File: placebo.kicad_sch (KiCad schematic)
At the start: 15 parts

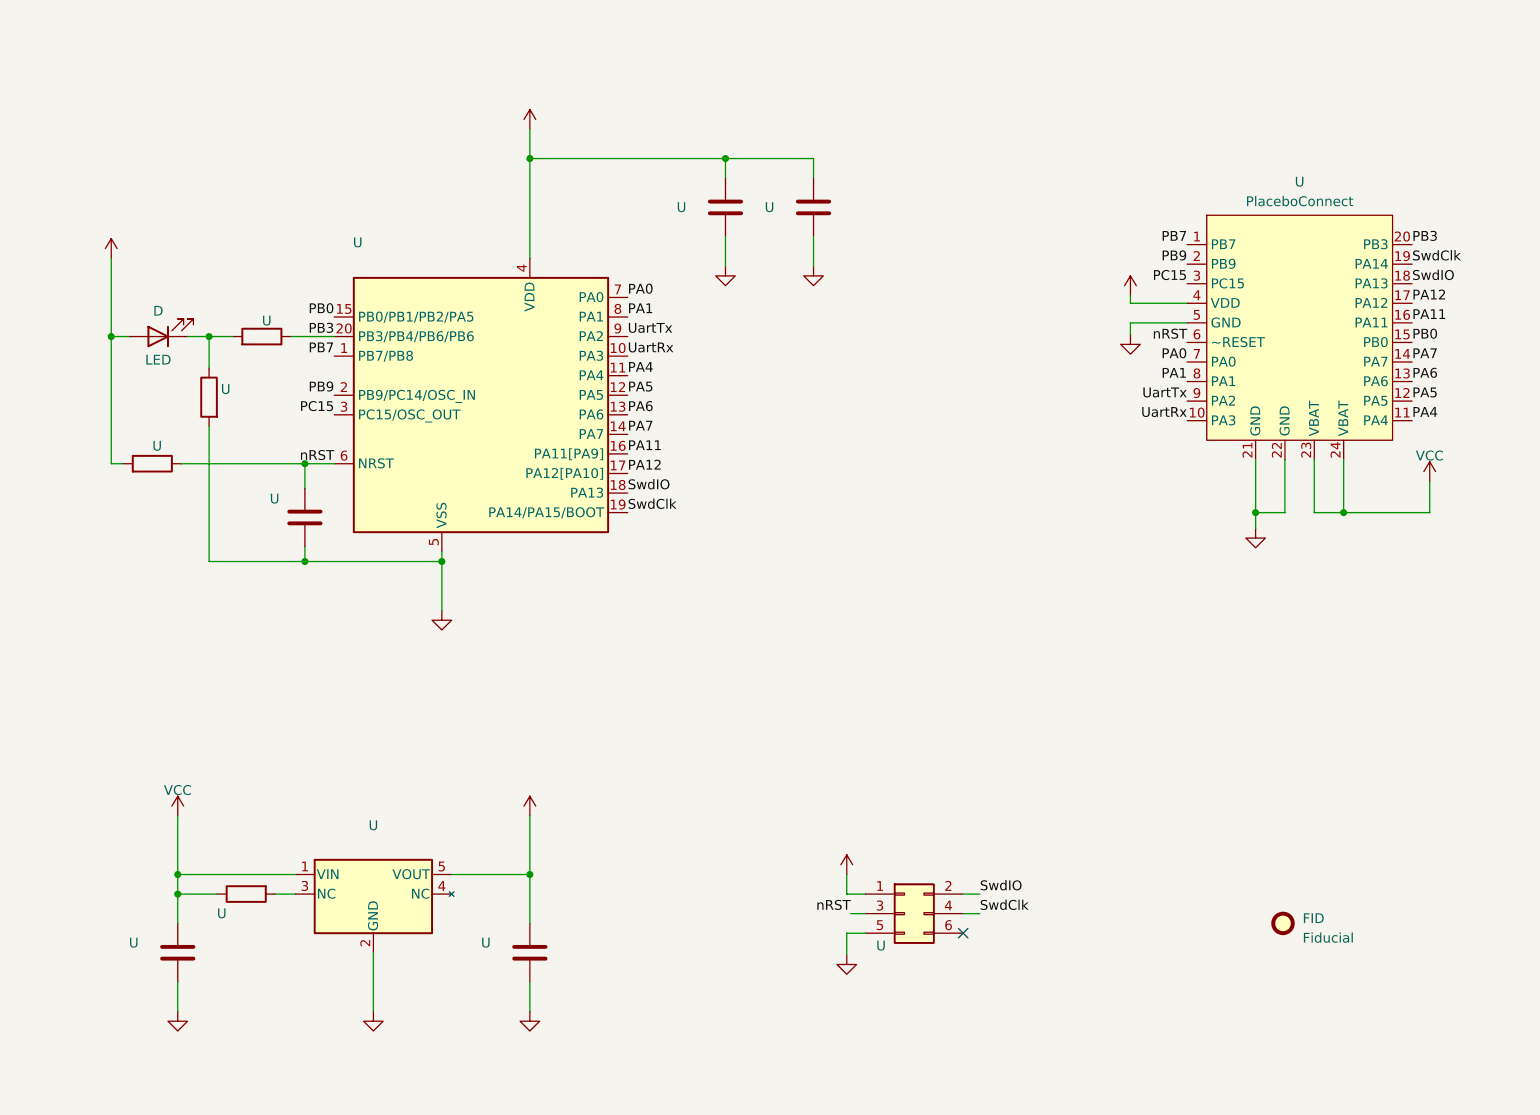
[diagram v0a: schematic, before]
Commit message: rev.0x7
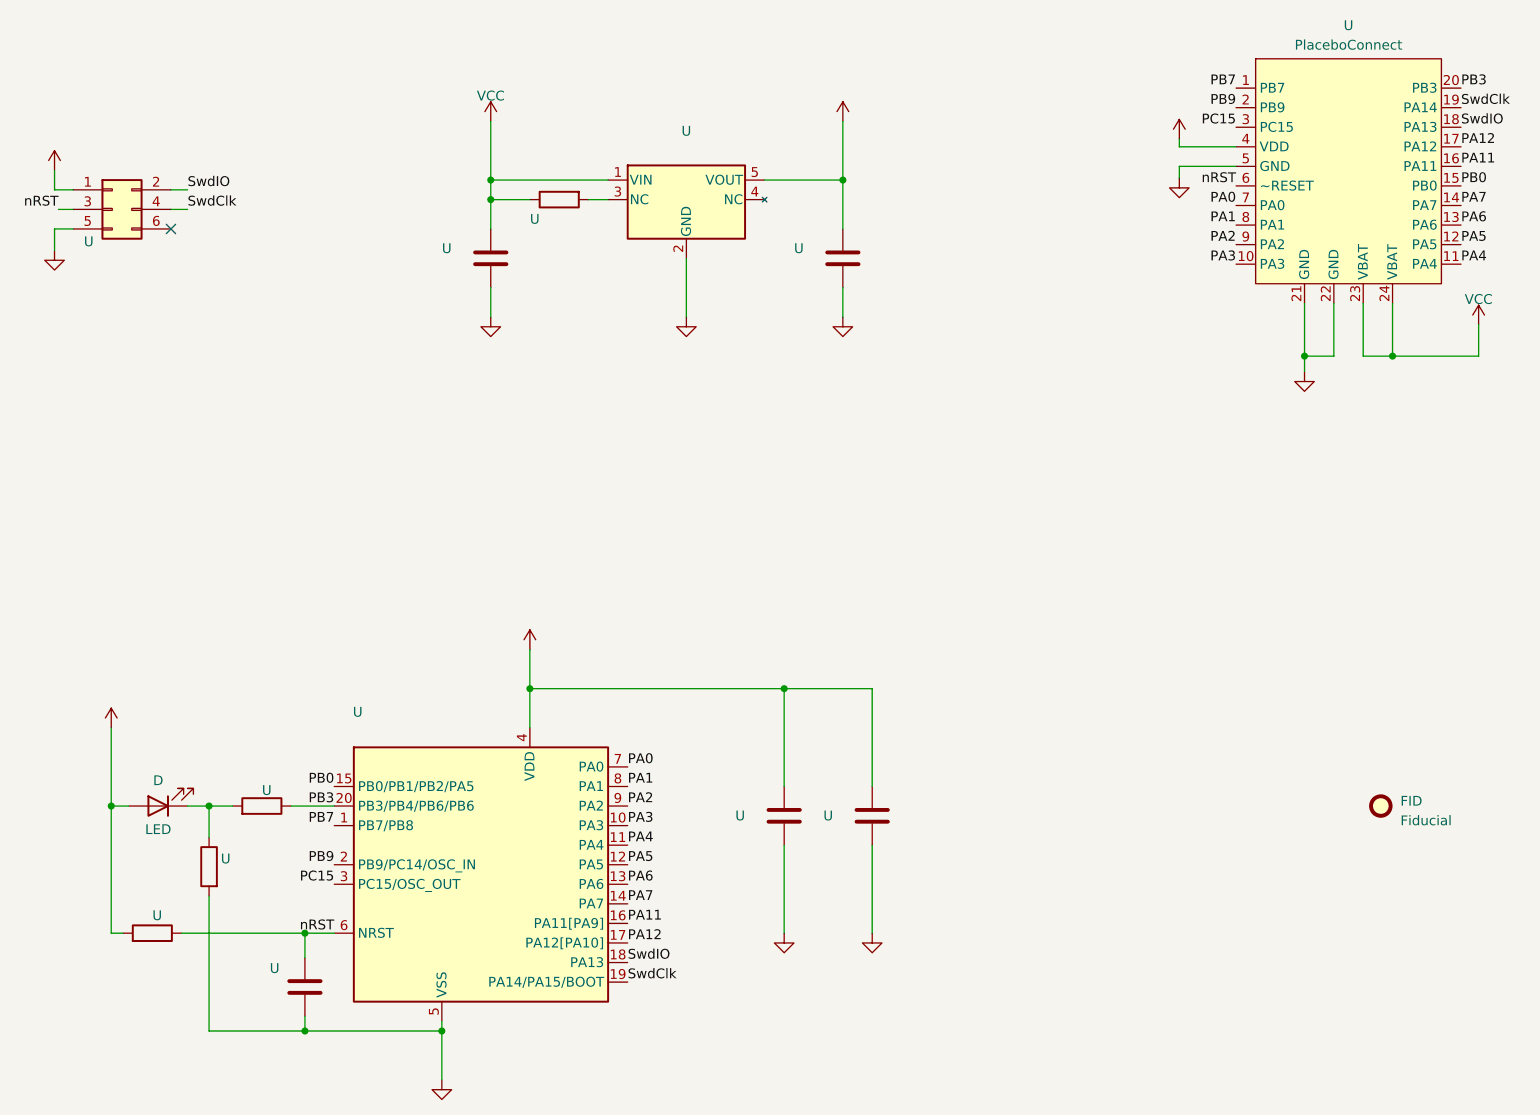
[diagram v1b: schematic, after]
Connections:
- net UartRx renamed PA3
- net UartTx renamed PA2
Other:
- moved on the sheet: D, FID, U
